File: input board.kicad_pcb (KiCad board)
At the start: 2 copper layers, 149.9 x 148.6 mm, 78 parts, among them J1 Conn_01x05_Female, J10 Conn_01x05_Female, J11 Conn_01x04_Female, J12 MCU_LEFT_LEGS, J13 MCU_RIGHT_LEGS, J2 Conn_01x05_Female, J3 Conn_01x05_Female, J4 Conn_01x05_Female, J5 Conn_01x05_Female, J6 Conn_01x05_Female, J7 Conn_01x05_Female, J8 Conn_01x05_Female, J9 Conn_01x05_Female

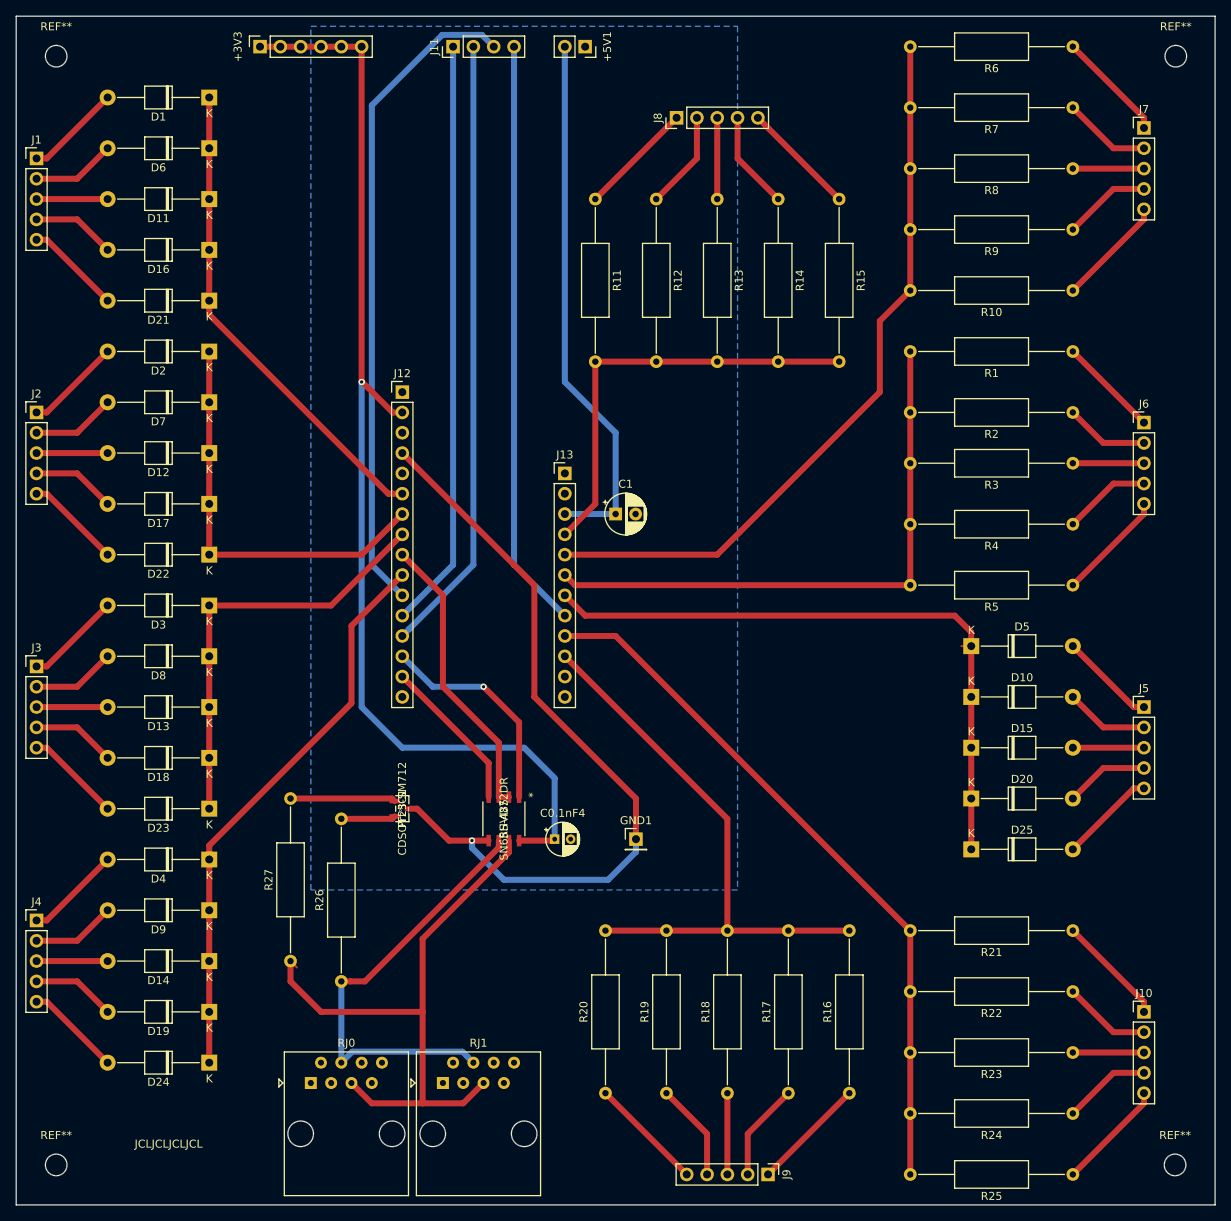
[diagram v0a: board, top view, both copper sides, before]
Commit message: Updated PCB and gbr files
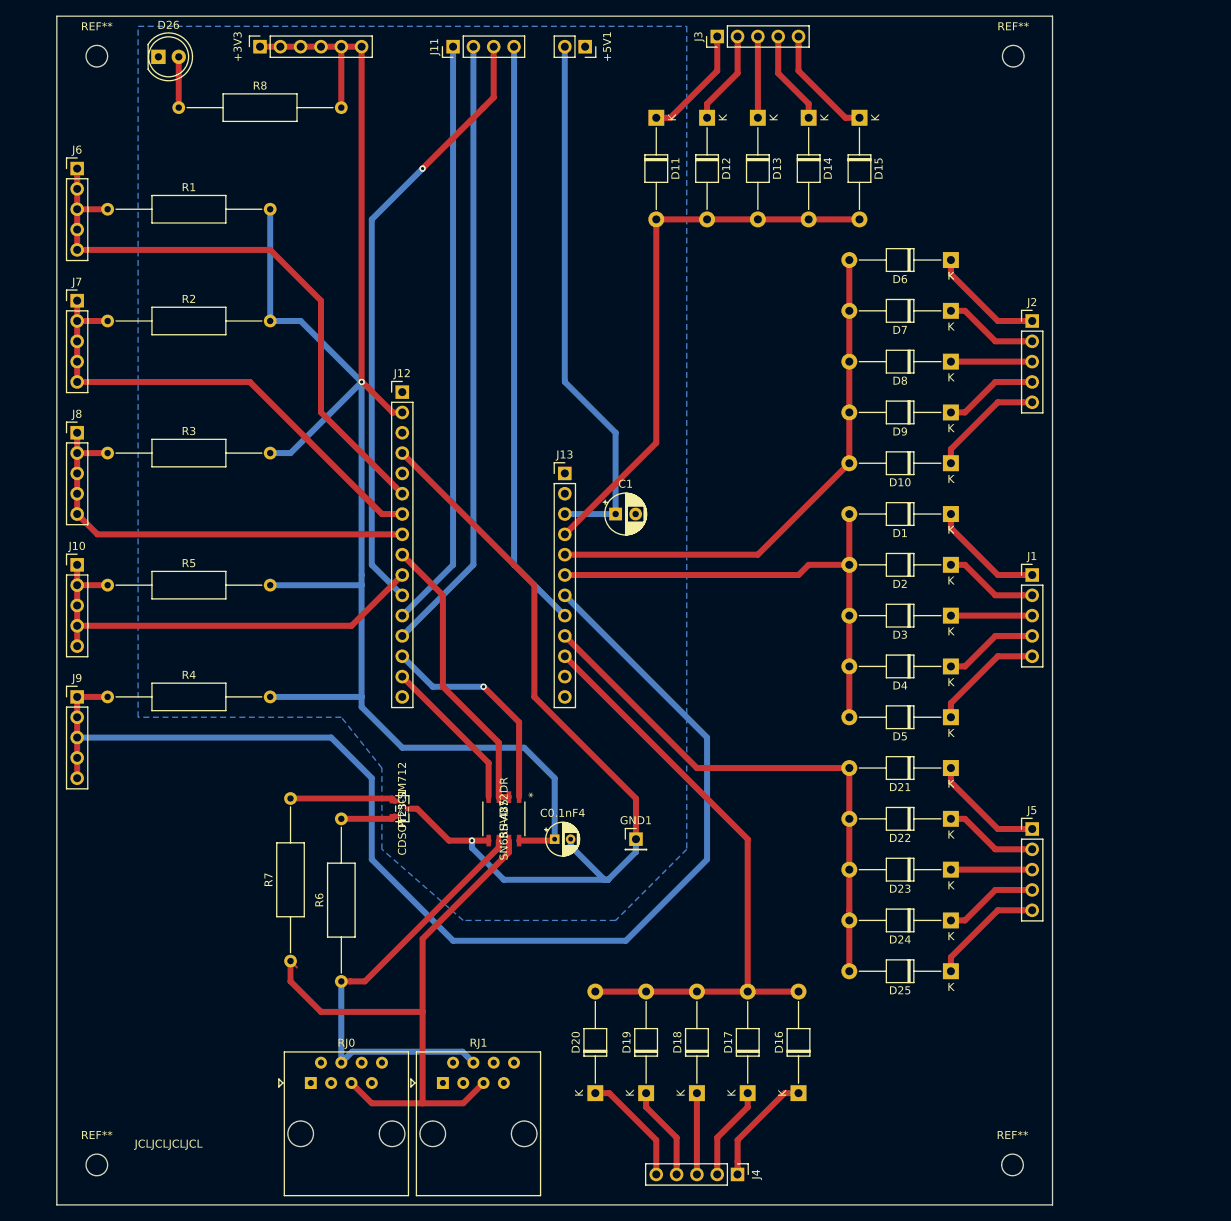
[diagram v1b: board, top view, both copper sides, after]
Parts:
- removed R10, R11, R12, R13, R14, R15, R16, R17, R18, R19, R20, R21, R22, R23, R24, R25, R9: 220, Resistor_THT:R_Axial_DIN0309_L9.0mm_D3.2mm_P20.32mm_Horizontal
- removed the R6 at (189.2, 21.6)
- removed the R7 at (189.2, 29.2)
- added D26: LED, LED_THT:LED_D5.0mm, F.Cu at (74.9, 22.9)
- R1, R2, R3, R4, R5: value 220 -> 10k
- R8: value 220 -> 470
- moved J10 144.6 mm to (64.8, 86.4)
- moved J6 137.1 mm to (64.8, 36.8)
- moved J7 135.1 mm to (64.8, 53.3)
- moved J1 134.9 mm to (184.2, 87.6)
- moved D14 129.3 mm to (156.2, 30.5), turned to 270 degrees
- moved D16 128.6 mm to (154.9, 152.4), turned to 90 degrees
- moved J2 125.0 mm to (184.2, 55.9)
- moved R4 122.6 mm to (68.6, 102.9), turned to 0 degrees
- moved R1 122.0 mm to (68.6, 41.9), turned to 0 degrees
- moved R2 121.2 mm to (68.6, 55.9), turned to 0 degrees
- moved R3 120.7 mm to (68.6, 72.4), turned to 0 degrees
- moved R5 120.6 mm to (68.6, 88.9), turned to 0 degrees
- moved J3 115.9 mm to (144.8, 20.3), turned to 90 degrees
- moved R8 112.0 mm to (77.5, 29.2), turned to 0 degrees
- moved D9 111.7 mm to (174.0, 67.3)
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- renumbered R26 to R6, R27 to R7
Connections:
- D1 pad 1: /A1 -> Net-(D1-Pad1)
- D1 pad 2: /101 -> /D11
- D10 pad 1: /D10 -> Net-(D10-Pad1)
- D10 pad 2: /205 -> /D12
- D11 pad 1: /A1 -> Net-(D11-Pad1)
- D11 pad 2: /301 -> /D13
- D12 pad 1: /A2 -> Net-(D12-Pad1)
- D12 pad 2: /302 -> /D13
- D13 pad 1: /A3 -> Net-(D13-Pad1)
- D13 pad 2: /303 -> /D13
- D14 pad 1: /A5 -> Net-(D14-Pad1)
- D14 pad 2: /304 -> /D13
- D15 pad 1: /D10 -> Net-(D15-Pad1)
- D15 pad 2: /305 -> /D13
- D16 pad 1: /A1 -> Net-(D16-Pad1)
- D16 pad 2: /401 -> /D5
- D17 pad 1: /A2 -> Net-(D17-Pad1)
- D17 pad 2: /402 -> /D5
- D18 pad 1: /A3 -> Net-(D18-Pad1)
- D18 pad 2: /403 -> /D5
- D19 pad 1: /A5 -> Net-(D19-Pad1)
- D19 pad 2: /404 -> /D5
- D2 pad 1: /A2 -> Net-(D2-Pad1)
- D2 pad 2: /102 -> /D11
- D20 pad 1: /D10 -> Net-(D20-Pad1)
- D20 pad 2: /405 -> /D5
- D21 pad 1: /A1 -> Net-(D21-Pad1)
- D21 pad 2: /501 -> /D6
- D22 pad 1: /A2 -> Net-(D22-Pad1)
- D22 pad 2: /502 -> /D6
- D23 pad 1: /A3 -> Net-(D23-Pad1)
- D23 pad 2: /503 -> /D6
- D24 pad 1: /A5 -> Net-(D24-Pad1)
- D24 pad 2: /504 -> /D6
- D25 pad 1: /D10 -> Net-(D25-Pad1)
- D25 pad 2: /505 -> /D6
- D3 pad 1: /A3 -> Net-(D3-Pad1)
- D3 pad 2: /103 -> /D11
- D4 pad 1: /A5 -> Net-(D4-Pad1)
- D4 pad 2: /104 -> /D11
- D5 pad 1: /D10 -> Net-(D5-Pad1)
- D5 pad 2: /105 -> /D11
- D6 pad 1: /A1 -> Net-(D6-Pad1)
- D6 pad 2: /201 -> /D12
- D7 pad 1: /A2 -> Net-(D7-Pad1)
- D7 pad 2: /202 -> /D12
- D8 pad 1: /A3 -> Net-(D8-Pad1)
- D8 pad 2: /203 -> /D12
- D9 pad 1: /A5 -> Net-(D9-Pad1)
- D9 pad 2: /204 -> /D12
- J1 pad 1: /101 -> Net-(D1-Pad1)
- J1 pad 2: /201 -> Net-(D2-Pad1)
- J1 pad 3: /301 -> Net-(D3-Pad1)
- J1 pad 4: /401 -> Net-(D4-Pad1)
- J1 pad 5: /501 -> Net-(D5-Pad1)
- J10 pad 1: /501 -> /A5
- J10 pad 2: /502 -> /A5
- J10 pad 3: /503 -> /A5
- J10 pad 4: /504 -> /A5
- J10 pad 5: /505 -> /A5
- J2 pad 1: /102 -> Net-(D6-Pad1)
- J2 pad 2: /202 -> Net-(D7-Pad1)
- J2 pad 3: /302 -> Net-(D8-Pad1)
- J2 pad 4: /402 -> Net-(D9-Pad1)
- J2 pad 5: /502 -> Net-(D10-Pad1)
- J3 pad 1: /103 -> Net-(D11-Pad1)
- J3 pad 2: /203 -> Net-(D12-Pad1)
- J3 pad 3: /303 -> Net-(D13-Pad1)
- J3 pad 4: /403 -> Net-(D14-Pad1)
- J3 pad 5: /503 -> Net-(D15-Pad1)
- J4 pad 1: /104 -> Net-(D16-Pad1)
- J4 pad 2: /204 -> Net-(D17-Pad1)
- J4 pad 3: /304 -> Net-(D18-Pad1)
- J4 pad 4: /404 -> Net-(D19-Pad1)
- J4 pad 5: /504 -> Net-(D20-Pad1)
- J5 pad 1: /105 -> Net-(D21-Pad1)
- J5 pad 2: /205 -> Net-(D22-Pad1)
- J5 pad 3: /305 -> Net-(D23-Pad1)
- J5 pad 4: /405 -> Net-(D24-Pad1)
- J5 pad 5: /505 -> Net-(D25-Pad1)
- J6 pad 1: /101 -> /A1
- J6 pad 2: /102 -> /A1
- J6 pad 3: /103 -> /A1
- J6 pad 4: /104 -> /A1
- J6 pad 5: /105 -> /A1
- J7 pad 1: /201 -> /A2
- J7 pad 2: /202 -> /A2
- J7 pad 3: /203 -> /A2
- J7 pad 4: /204 -> /A2
- J7 pad 5: /205 -> /A2
- J8 pad 1: /301 -> /A3
- J8 pad 2: /302 -> /A3
- J8 pad 3: /303 -> /A3
- J8 pad 4: /304 -> /A3
- J8 pad 5: /305 -> /A3
- J9 pad 1: /401 -> /D10
- J9 pad 2: /402 -> /D10
- J9 pad 3: /403 -> /D10
- J9 pad 4: /404 -> /D10
- J9 pad 5: /405 -> /D10
- R1 pad 1: /101 -> /A1
- R1 pad 2: /D11 -> +3V3
- R2 pad 1: /102 -> /A2
- R2 pad 2: /D11 -> +3V3
- R3 pad 1: /103 -> /A3
- R3 pad 2: /D11 -> +3V3
- R4 pad 1: /104 -> /D10
- R4 pad 2: /D11 -> +3V3
- R5 pad 1: /105 -> /A5
- R5 pad 2: /D11 -> +3V3
- R8 pad 1: /203 -> Net-(D26-Pad2)
- R8 pad 2: /D12 -> +3V3
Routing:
- net +3V3: track 141.8 -> 216.0 mm
- net /D10: track 81.1 -> 153.8 mm
- net /D12: track 92.5 -> 65.7 mm
- net /105: track 25.9 -> 0.00 mm
- net /505: track 25.9 -> 0.00 mm
- net /501: track 25.9 -> 0.00 mm
- net /405: track 24.8 -> 0.00 mm
- net /401: track 24.8 -> 0.00 mm
- net /101: track 24.6 -> 0.00 mm
- net /205: track 24.3 -> 0.00 mm
- net /201: track 24.3 -> 0.00 mm
- net /305: track 23.3 -> 0.00 mm
- net /301: track 23.3 -> 0.00 mm
- net /502: track 23.0 -> 0.00 mm
- net /104: track 23.0 -> 0.00 mm
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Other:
- board size 149.9 x 148.6 mm -> 124.5 x 148.6 mm
